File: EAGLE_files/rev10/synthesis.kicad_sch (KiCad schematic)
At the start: 60 parts, among them J1 Conn_01x02_Pin, J18 110990030, SW1 B3F-1025, U23 INA2134UA, U24 INA2134UA, U28 OPA1642AIDR, U29 DRV135UA/2K5, U3 OPA1642AIDR

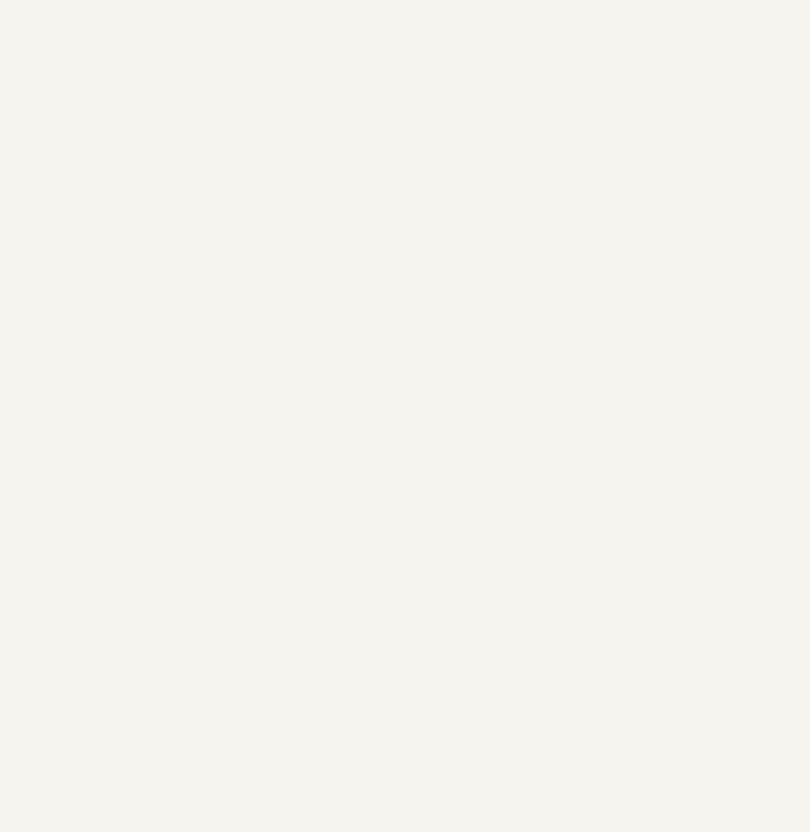
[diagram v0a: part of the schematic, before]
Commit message: working on 5 string version
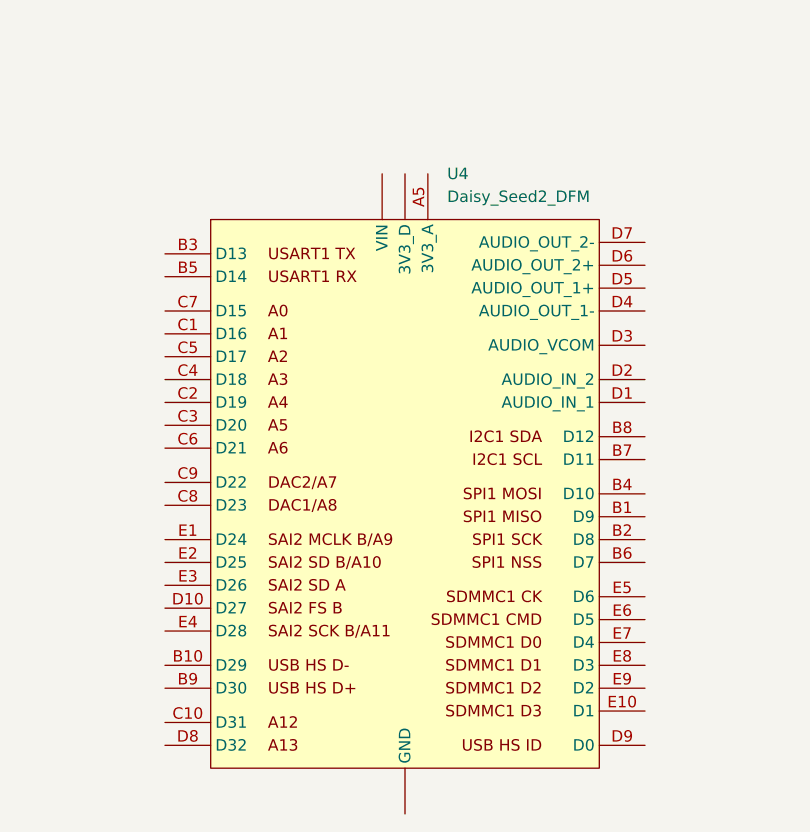
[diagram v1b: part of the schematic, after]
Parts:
- added U4: Daisy_Seed2_DFM, Snapeda:DAISY_PATCH_SM, symbol Snapeda:Daisy_Seed2_DFM
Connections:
- new net: U4.A1 (VIN), U4.A2 (VIN)
- new net: U4.A10 (GND), U4.A6 (GND), U4.A7 (GND), U4.A8 (GND), U4.A9 (GND)
- new net: U4.A3 (3V3_D), U4.A4 (3V3_D)
